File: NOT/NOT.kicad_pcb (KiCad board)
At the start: 2 copper layers, 17.8 x 17.8 mm, 6 parts

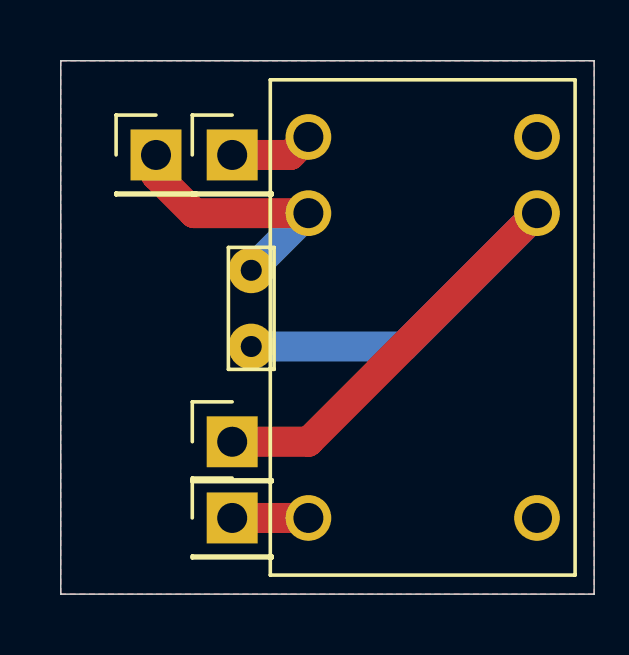
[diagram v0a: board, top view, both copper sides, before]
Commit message: Add files via upload
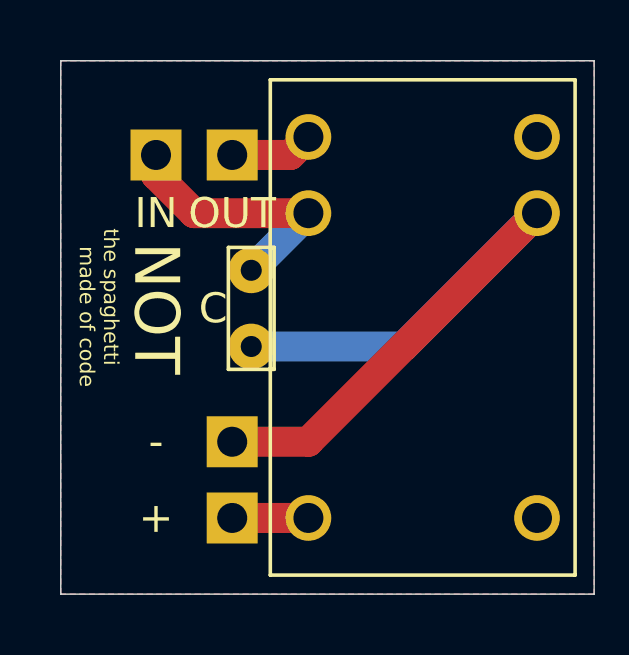
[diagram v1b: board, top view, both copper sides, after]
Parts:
- REF** (x4): moved to B.Cu

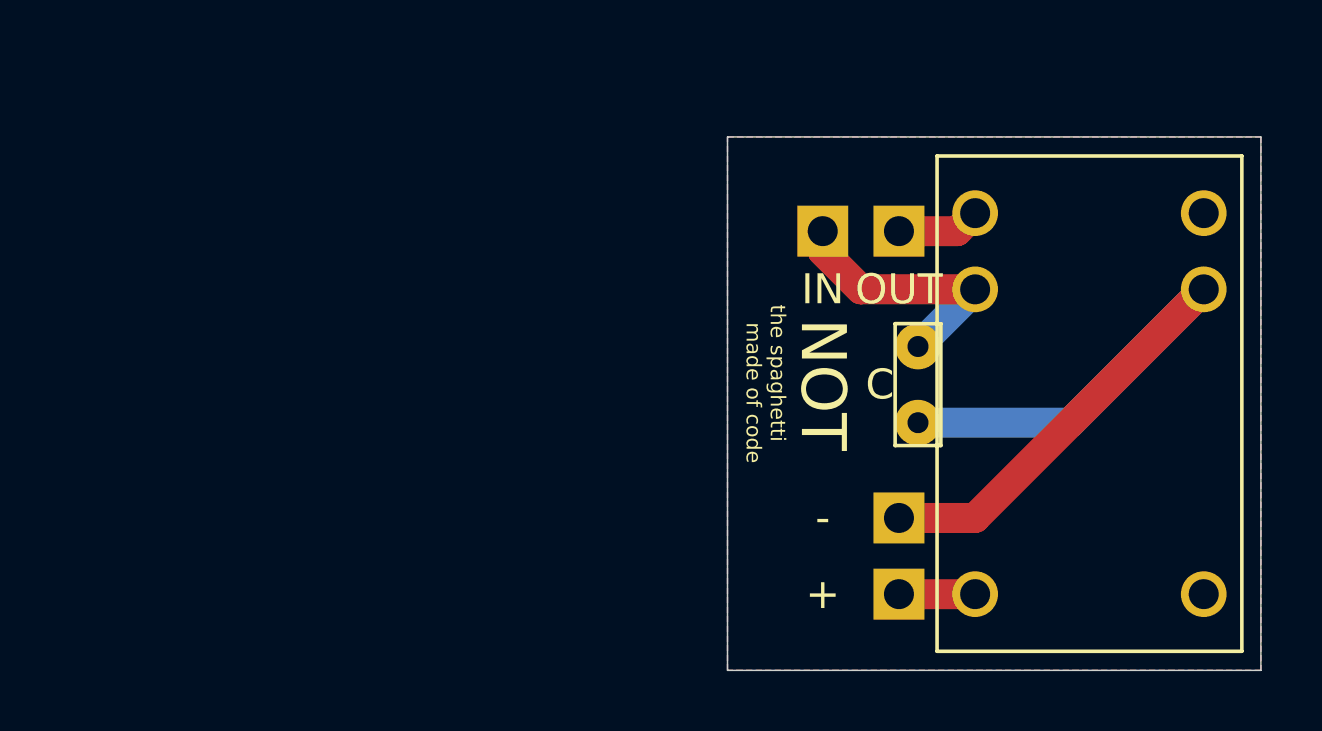
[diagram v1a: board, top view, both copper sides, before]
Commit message: Add files via upload
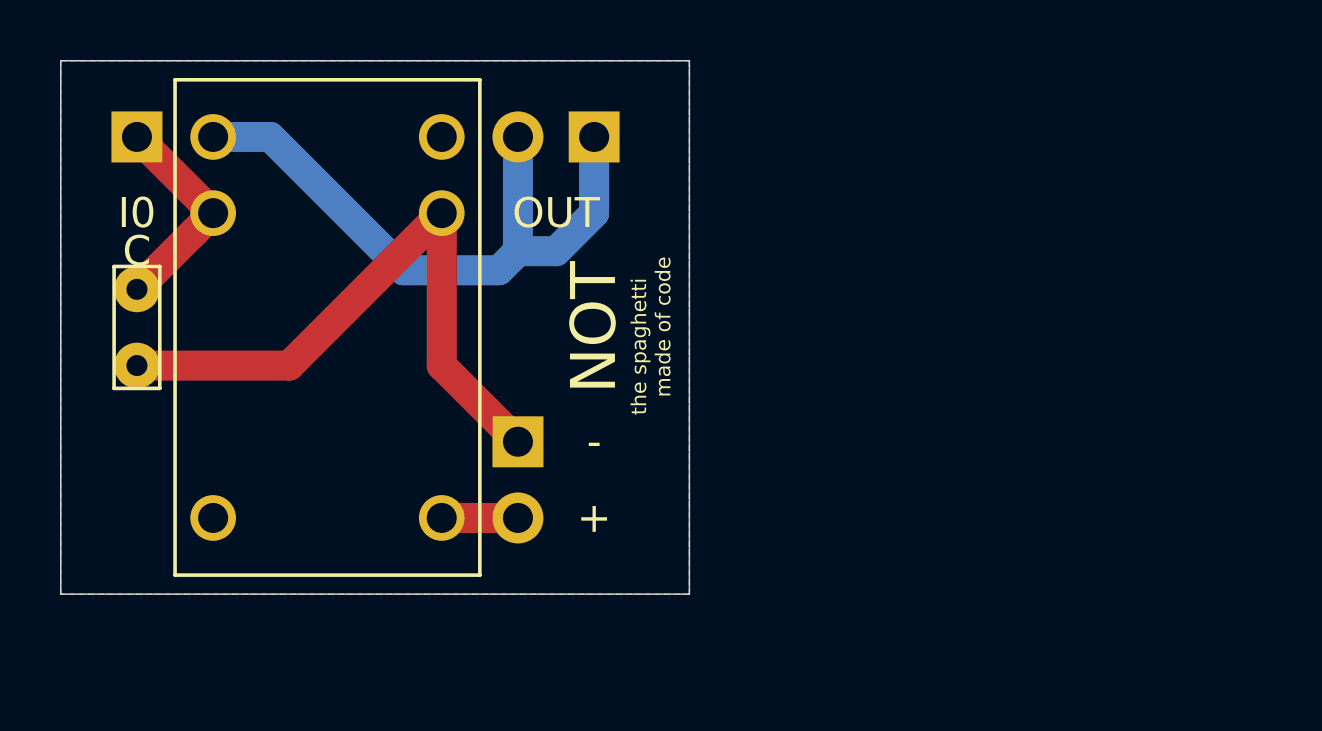
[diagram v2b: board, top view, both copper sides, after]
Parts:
- removed REF**: Condensor, MiyakeFootprintLib:Condensor
- removed REF** (x4): PinHeader_1x01_P2.54mm_Vertical, Connector_PinHeader_2.54mm:PinHeader_1x01_P2.54mm_Vertical
- removed REF**: 946H-1C-24D, MiyakeFootprintLib:946H-1C-24D
- added C1: C, MiyakeFootprintLib:Condensor, F.Cu at (104.1, 78.7)
- added J1: Conn_01x01, Connector_PinHeader_2.54mm:PinHeader_1x01_P2.54mm_Vertical, B.Cu at (104.1, 71.1)
- added J2: Conn_01x02, Connector_PinHeader_2.54mm:PinHeader_1x02_P2.54mm_Vertical, B.Cu at (119.4, 71.1)
- added J3: Conn_01x02, Connector_PinHeader_2.54mm:PinHeader_1x02_P2.54mm_Vertical, B.Cu at (116.8, 81.3)
- added SPDT1: 946H-1C-24D, MiyakeFootprintLib:946H-1C-24D, F.Cu at (111.8, 76.2)
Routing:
- net (no net): track 39.0 -> 0.00 mm
- net Net-(J2-Pad1): track 0.00 -> 21.7 mm
- net GND: track 0.00 -> 20.9 mm
- net Net-(C1-Pad2): track 0.00 -> 7.18 mm
- net +24V: track 0.00 -> 2.54 mm
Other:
- board size 17.8 x 17.8 mm -> 21 x 17.8 mm
- board text added: "I0"
- board text removed: "IN"
